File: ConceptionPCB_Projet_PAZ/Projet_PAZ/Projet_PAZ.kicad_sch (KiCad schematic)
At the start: 11 parts, among them J3 XT60-M, U1 BU33SD5WG-TR

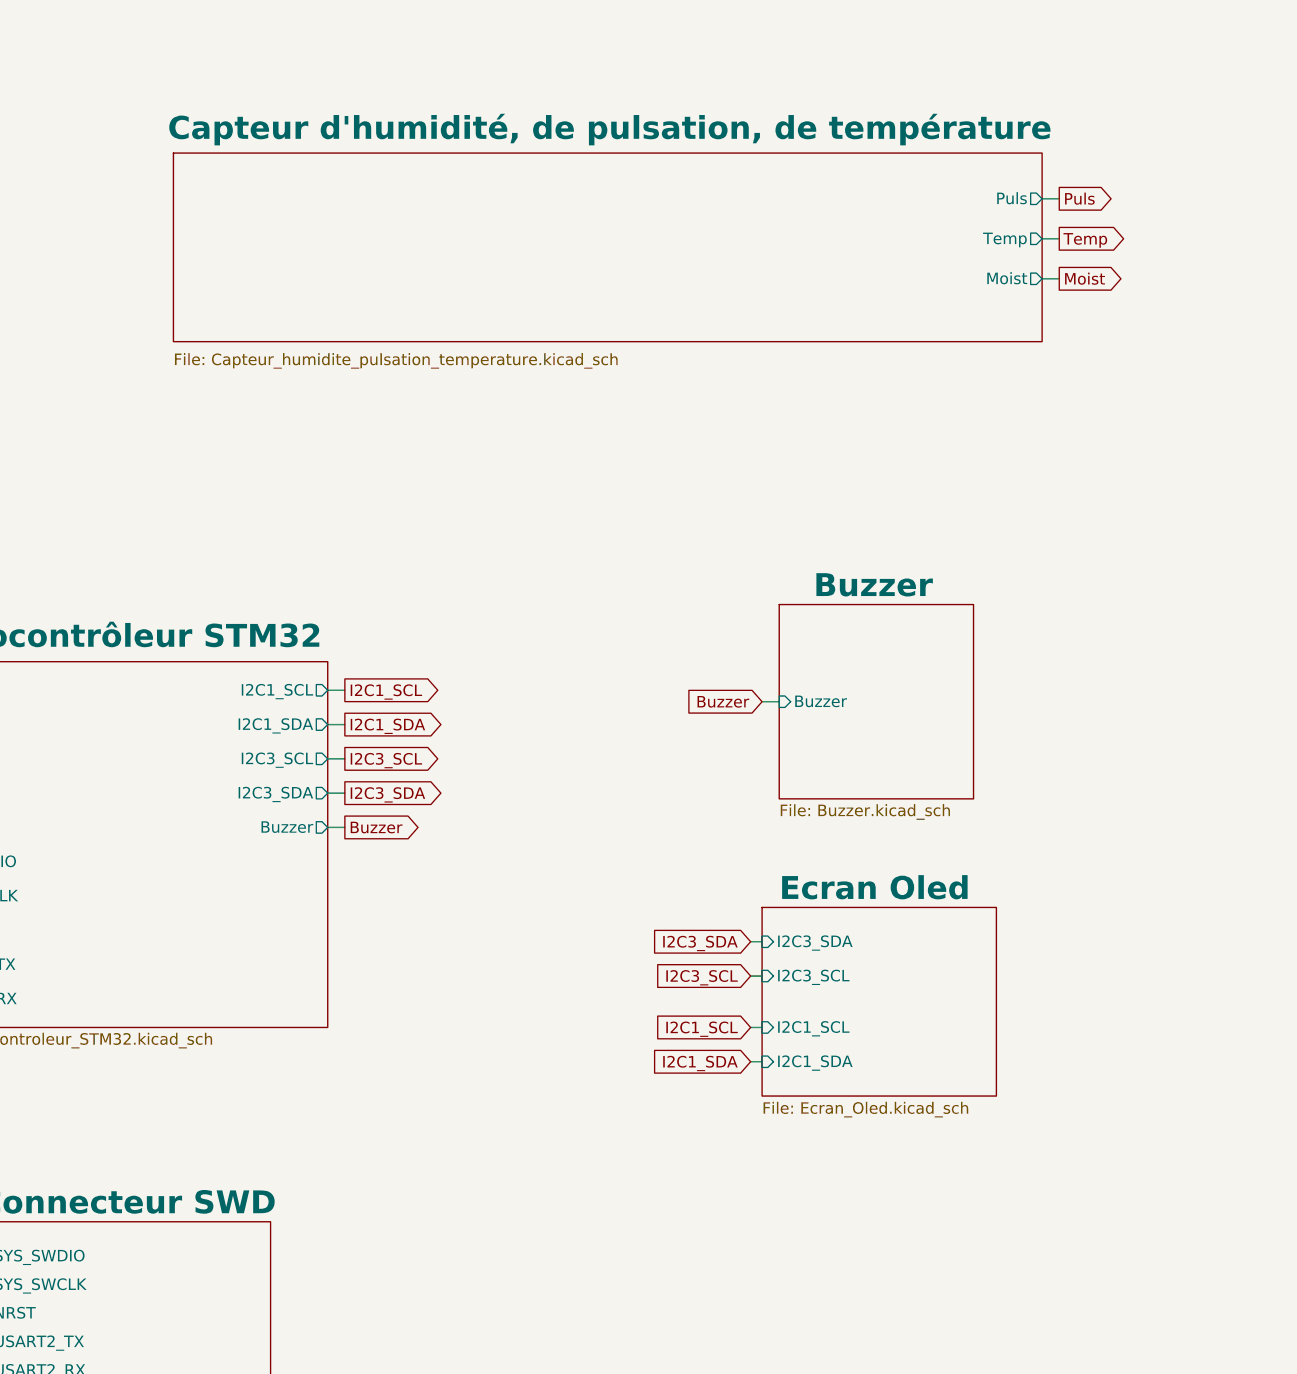
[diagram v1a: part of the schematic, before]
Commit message: Add files via upload
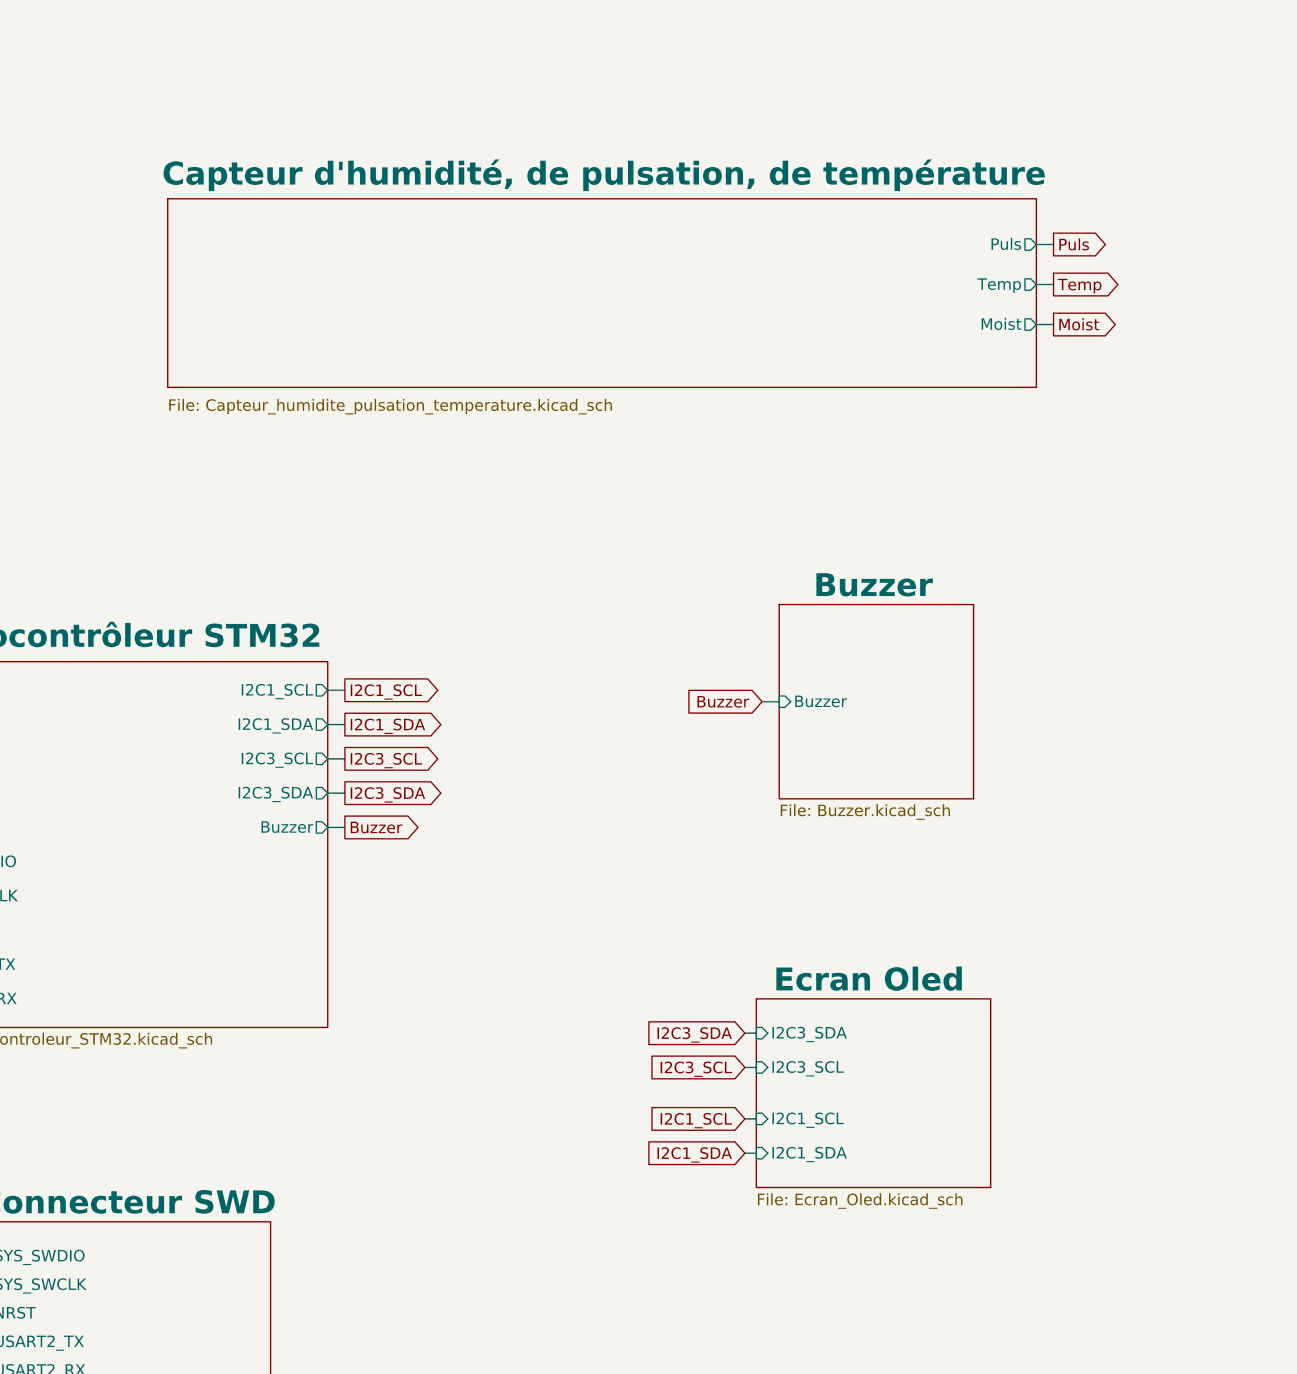
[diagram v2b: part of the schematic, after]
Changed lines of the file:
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@@
     (stroke (width 0) (type default))
   )
-  (wire (pts (xy 223.52 121.285) (xy 224.79 121.285))
+  (wire (pts (xy 222.885 131.445) (xy 224.155 131.445))
     (stroke (width 0) (type default))
   )
@@
     (stroke (width 0) (type default))
   )
-  (wire (pts (xy 223.52 130.81) (xy 224.79 130.81))
+  (wire (pts (xy 222.885 140.97) (xy 224.155 140.97))
     (stroke (width 0) (type default))
   )
@@
     (stroke (width 0) (type default))
   )
-  (wire (pts (xy 255.905 34.925) (xy 257.81 34.925))
+  (wire (pts (xy 255.27 40.005) (xy 257.175 40.005))
     (stroke (width 0) (type default))
   )
@@
     (stroke (width 0) (type default))
   )
-  (wire (pts (xy 223.52 117.475) (xy 224.79 117.475))
+  (wire (pts (xy 222.885 127.635) (xy 224.155 127.635))
     (stroke (width 0) (type default))
   )
@@
     (stroke (width 0) (type default))
   )
-  (wire (pts (xy 223.52 127) (xy 224.79 127))
+  (wire (pts (xy 222.885 137.16) (xy 224.155 137.16))
     (stroke (width 0) (type default))
   )
@@
     (stroke (width 0) (type default))
   )
-  (wire (pts (xy 255.905 39.37) (xy 257.81 39.37))
+  (wire (pts (xy 255.27 44.45) (xy 257.175 44.45))
     (stroke (width 0) (type default))
   )
@@
     (stroke (width 0) (type default))
   )
-  (wire (pts (xy 255.905 43.815) (xy 257.81 43.815))
+  (wire (pts (xy 255.27 48.895) (xy 257.175 48.895))
     (stroke (width 0) (type default))
   )
@@
     )
   )
-  (global_label "I2C1_SCL" (shape input) (at 223.52 127 180) (fields_autoplaced)
-    (effects (font (size 1.27 1.27)) (justify right))
-    (property "Intersheetrefs" "${INTERSHEET_REFS}" (at 211.7658 127 0)
+  (global_label "I2C1_SCL" (shape input) (at 222.885 137.16 180) (fields_autoplaced)
+    (effects (font (size 1.27 1.27)) (justify right))
+    (property "Intersheetrefs" "${INTERSHEET_REFS}" (at 211.1308 137.16 0)
       (effects (font (size 1.27 1.27)) (justify right) hide)
     )
@@
     )
   )
-  (global_label "I2C3_SCL" (shape input) (at 223.52 121.285 180) (fields_autoplaced)
-    (effects (font (size 1.27 1.27)) (justify right))
-    (property "Intersheetrefs" "${INTERSHEET_REFS}" (at 211.7658 121.285 0)
-      (effects (font (size 1.27 1.27)) (justify right) hide)
-    )
-  )
-  (global_label "I2C3_SDA" (shape input) (at 223.52 117.475 180) (fields_autoplaced)
-    (effects (font (size 1.27 1.27)) (justify right))
-    (property "Intersheetrefs" "${INTERSHEET_REFS}" (at 211.7053 117.475 0)
-      (effects (font (size 1.27 1.27)) (justify right) hide)
-    )
-  )
-  (global_label "Temp" (shape output) (at 257.81 39.37 0) (fields_autoplaced)
+  (global_label "I2C3_SCL" (shape input) (at 222.885 131.445 180) (fields_autoplaced)
+    (effects (font (size 1.27 1.27)) (justify right))
+    (property "Intersheetrefs" "${INTERSHEET_REFS}" (at 211.1308 131.445 0)
+      (effects (font (size 1.27 1.27)) (justify right) hide)
+    )
+  )
+  (global_label "I2C3_SDA" (shape input) (at 222.885 127.635 180) (fields_autoplaced)
+    (effects (font (size 1.27 1.27)) (justify right))
+    (property "Intersheetrefs" "${INTERSHEET_REFS}" (at 211.0703 127.635 0)
+      (effects (font (size 1.27 1.27)) (justify right) hide)
+    )
+  )
+  (global_label "Temp" (shape output) (at 257.175 44.45 0) (fields_autoplaced)
     (effects (font (size 1.27 1.27)) (justify left))
-    (property "Intersheetrefs" "${INTERSHEET_REFS}" (at 265.6937 39.37 0)
+    (property "Intersheetrefs" "${INTERSHEET_REFS}" (at 265.0587 44.45 0)
       (effects (font (size 1.27 1.27)) (justify left) hide)
     )
   )
-  (global_label "I2C1_SDA" (shape input) (at 223.52 130.81 180) (fields_autoplaced)
-    (effects (font (size 1.27 1.27)) (justify right))
-    (property "Intersheetrefs" "${INTERSHEET_REFS}" (at 211.7053 130.81 0)
+  (global_label "I2C1_SDA" (shape input) (at 222.885 140.97 180) (fields_autoplaced)
+    (effects (font (size 1.27 1.27)) (justify right))
+    (property "Intersheetrefs" "${INTERSHEET_REFS}" (at 211.0703 140.97 0)
       (effects (font (size 1.27 1.27)) (justify right) hide)
     )
@@
     )
   )
-  (global_label "Moist" (shape output) (at 257.81 43.815 0) (fields_autoplaced)
+  (global_label "Moist" (shape output) (at 257.175 48.895 0) (fields_autoplaced)
     (effects (font (size 1.27 1.27)) (justify left))
-    (property "Intersheetrefs" "${INTERSHEET_REFS}" (at 265.7542 43.815 0)
+    (property "Intersheetrefs" "${INTERSHEET_REFS}" (at 265.1192 48.895 0)
       (effects (font (size 1.27 1.27)) (justify left) hide)
     )
@@
     )
   )
-  (global_label "Puls" (shape output) (at 257.81 34.925 0) (fields_autoplaced)
+  (global_label "Puls" (shape output) (at 257.175 40.005 0) (fields_autoplaced)
     (effects (font (size 1.27 1.27)) (justify left))
-    (property "Intersheetrefs" "${INTERSHEET_REFS}" (at 264.9075 34.925 0)
+    (property "Intersheetrefs" "${INTERSHEET_REFS}" (at 264.2725 40.005 0)
       (effects (font (size 1.27 1.27)) (justify left) hide)
     )
@@
     )
   )
-  (sheet (at 224.79 113.665) (size 26.035 20.955)
+  (sheet (at 224.155 123.825) (size 26.035 20.955)
     (stroke (width 0.1524) (type solid))
     (fill (color 0 0 0 0.0000))
-    (property "Sheetname" "Ecran Oled" (at 226.695 113.03 0)
+    (property "Sheetname" "Ecran Oled" (at 226.06 123.19 0)
       (effects (font (size 2.54 2.54) bold) (justify left bottom))
     )
-    (property "Sheetfile" "Ecran_Oled.kicad_sch" (at 224.79 135.255 0)
+    (property "Sheetfile" "Ecran_Oled.kicad_sch" (at 224.155 145.415 0)
       (effects (font (size 1.27 1.27)) (justify left top))
     )
-    (pin "I2C3_SDA" input (at 224.79 117.475 180)
-      (effects (font (size 1.27 1.27)) (justify left))
-    )
-    (pin "I2C3_SCL" input (at 224.79 121.285 180)
-      (effects (font (size 1.27 1.27)) (justify left))
-    )
-    (pin "I2C1_SCL" input (at 224.79 127 180)
-      (effects (font (size 1.27 1.27)) (justify left))
-    )
-    (pin "I2C1_SDA" input (at 224.79 130.81 180)
+    (pin "I2C3_SDA" input (at 224.155 127.635 180)
+      (effects (font (size 1.27 1.27)) (justify left))
+    )
+    (pin "I2C3_SCL" input (at 224.155 131.445 180)
+      (effects (font (size 1.27 1.27)) (justify left))
+    )
+    (pin "I2C1_SCL" input (at 224.155 137.16 180)
+      (effects (font (size 1.27 1.27)) (justify left))
+    )
+    (pin "I2C1_SDA" input (at 224.155 140.97 180)
       (effects (font (size 1.27 1.27)) (justify left))
     )
@@
     )
   )
-  (sheet (at 159.385 29.845) (size 96.52 20.955)
+  (sheet (at 158.75 34.925) (size 96.52 20.955)
     (stroke (width 0.1524) (type solid))
     (fill (color 0 0 0 0.0000))
-    (property "Sheetname" "Capteur d'humidité, de pulsation, de température" (at 158.75 28.575 0)
+    (property "Sheetname" "Capteur d'humidité, de pulsation, de température" (at 158.115 33.655 0)
       (effects (font (size 2.54 2.54) bold (color 0 132 132 1)) (justify left bottom))
     )
-    (property "Sheetfile" "Capteur_humidite_pulsation_temperature.kicad_sch" (at 159.385 52.07 0)
+    (property "Sheetfile" "Capteur_humidite_pulsation_temperature.kicad_sch" (at 158.75 57.15 0)
       (effects (font (size 1.27 1.27)) (justify left top))
     )
-    (pin "Puls" output (at 255.905 34.925 0)
+    (pin "Puls" output (at 255.27 40.005 0)
       (effects (font (size 1.27 1.27)) (justify right))
     )
-    (pin "Temp" output (at 255.905 39.37 0)
+    (pin "Temp" output (at 255.27 44.45 0)
       (effects (font (size 1.27 1.27)) (justify right))
     )
-    (pin "Moist" output (at 255.905 43.815 0)
+    (pin "Moist" output (at 255.27 48.895 0)
       (effects (font (size 1.27 1.27)) (justify right))
     )
